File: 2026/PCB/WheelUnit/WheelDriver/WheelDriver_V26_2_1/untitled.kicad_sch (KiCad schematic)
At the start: 63 parts, among them SW2 SW_MEC_5E, SW3 SW_MEC_5E, U7 MAX3051

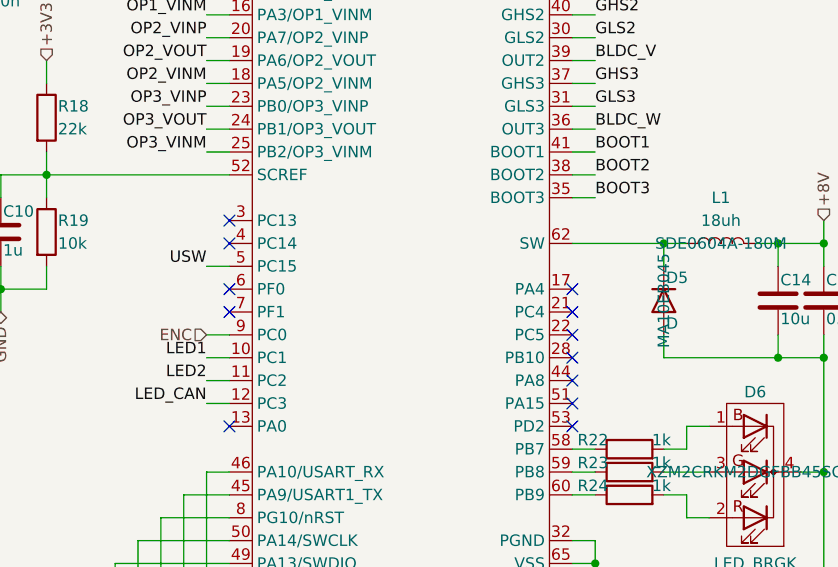
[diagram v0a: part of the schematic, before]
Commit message: ん、STPIN??周辺の配置だいたい終わり＆早く寝ましょう
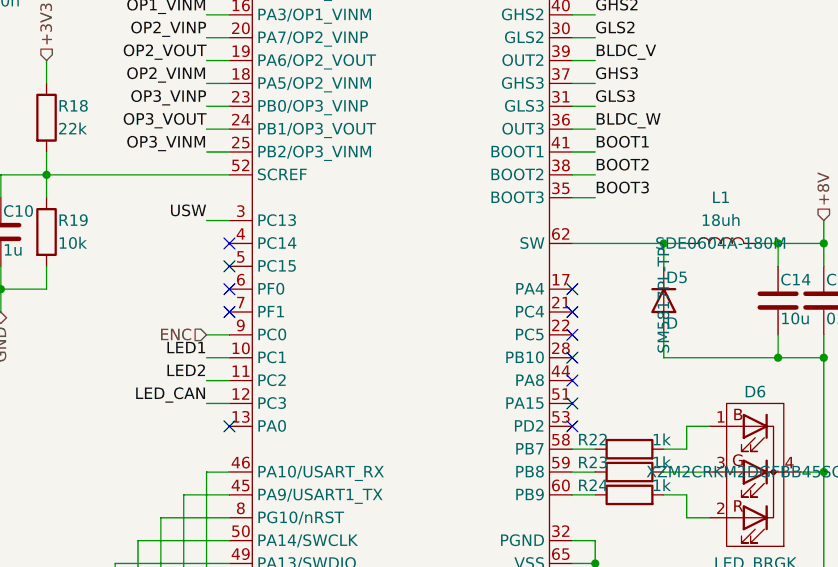
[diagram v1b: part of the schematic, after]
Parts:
- D5: footprint WheelUnit_LIB_FTP:MA10EB045 -> Diode_SMD:D_SOD-123F
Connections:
- net USW: now also MCU1.3 (PC13); no longer MCU1.5 (PC15)
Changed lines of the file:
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@@
 	)
 	(no_connect
-		(at 68.58 81.28)
-	)
-	(no_connect
 		(at 106.68 40.64)
 	)
@@
 	)
 	(no_connect
+		(at 68.58 86.36)
+	)
+	(no_connect
 		(at 106.68 101.6)
 	)
@@
 	(wire
 		(pts
-			(xy 66.04 86.36) (xy 68.58 86.36)
+			(xy 66.04 81.28) (xy 68.58 81.28)
 		)
 		(stroke
@@
 	)
 	(label "USW"
-		(at 66.04 86.36 180)
+		(at 66.04 81.28 180)
 		(effects
 			(font
@@
 			)
 		)
-		(property "Footprint" "WheelUnit_LIB_FTP:MA10EB045"
+		(property "Footprint" "Diode_SMD:D_SOD-123F"
 			(at 116.84 90.17 0)
 			(effects
@@
 			)
 		)
-		(property "Description" "MA10EB045"
+		(property "Description" "SM5817PL-TP"
 			(at 116.84 90.17 0)
 			(effects
